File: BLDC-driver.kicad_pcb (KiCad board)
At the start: 2 copper layers, 55.9 x 56 mm, 60 parts, among them J1 Conn_01x06, J2 Conn_01x06, Q1 FDMS86550, Q2 FDMS86550, Q3 FDMS86550, Q4 FDMS86550, Q5 FDMS86550, Q6 FDMS86550, U1 ADP3120A, U2 STM32F103C8Tx, U3 AS5600, U4 ADP3120A, U5 ADP3120A, U6 MP2359, U7 MIC5504-3.3YM5

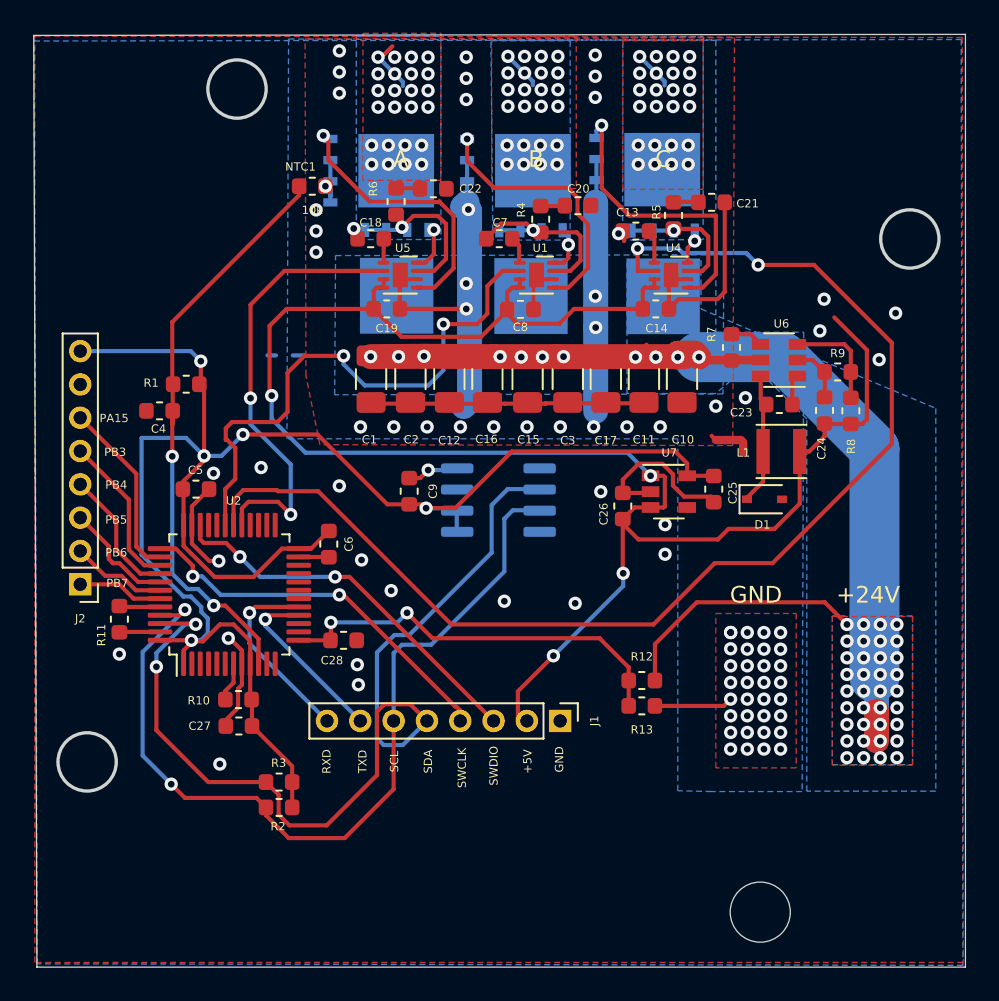
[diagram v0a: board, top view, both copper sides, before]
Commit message: Latest
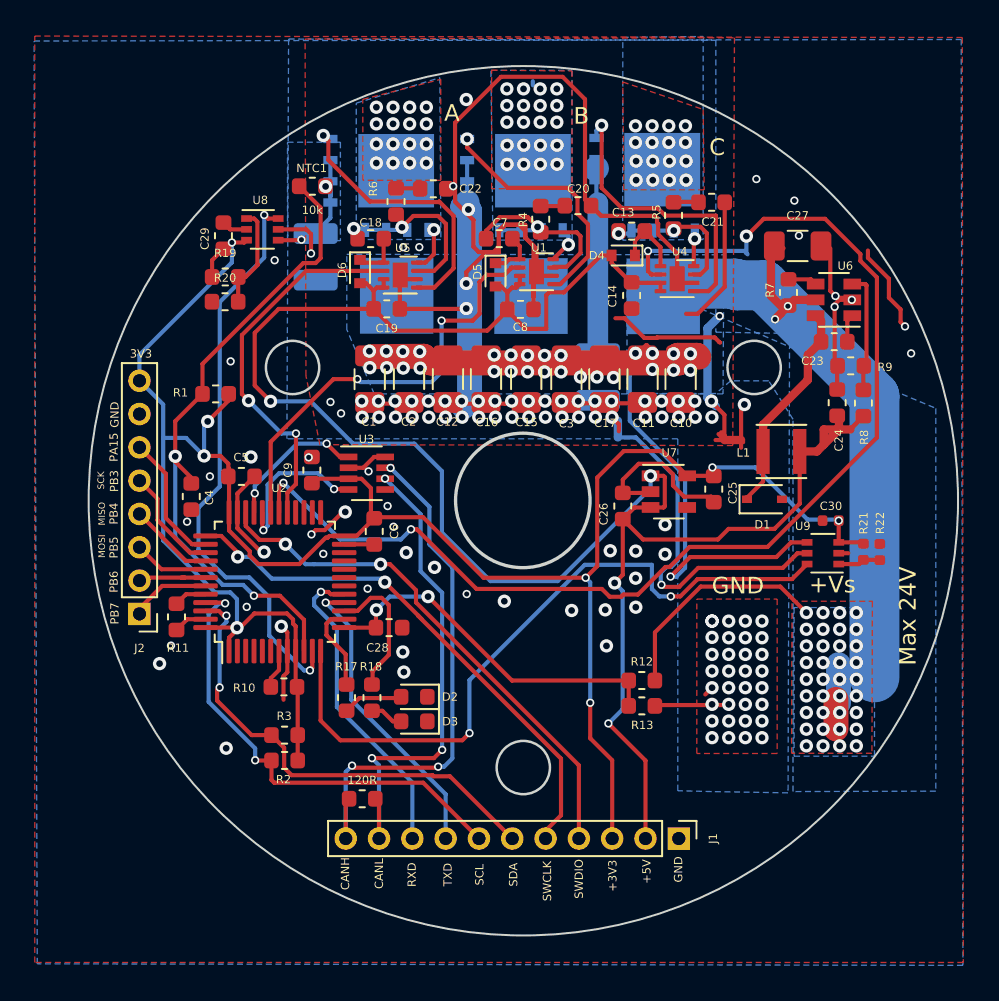
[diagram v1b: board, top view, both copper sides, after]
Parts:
- added C29: 100nF, Capacitor_SMD:C_0603_1608Metric, F.Cu at (178.7, 107.2)
- added C30: 100nF, Capacitor_SMD:C_0402_1005Metric, F.Cu at (215.2, 124.3)
- added D2: LED, LED_SMD:LED_0603_1608Metric, F.Cu at (190.2, 134.9)
- added D3: LED, LED_SMD:LED_0603_1608Metric, F.Cu at (190.2, 136.4)
- added D4: 30V, Diode_SMD:D_SOD-523, F.Cu at (202.7, 108.4)
- added D5: 30V, Diode_SMD:D_SOD-523, F.Cu at (195.0, 109.6)
- added D6: 30V, Diode_SMD:D_SOD-523, F.Cu at (186.9, 109.4)
- added NT2: Net-Tie_2, NetTie:NetTie-2_SMD_Pad0.5mm, B.Cu at (202.4, 118.8)
- added R14: 0.001, Resistor_SMD:R_1210_3225Metric, B.Cu at (184.3, 108.5)
- added R15: 0.001, Resistor_SMD:R_1210_3225Metric, B.Cu at (201.2, 115.7)
- added R16: 120R, Resistor_SMD:R_0603_1608Metric, F.Cu at (187.0, 141.0)
- added R17: 1k, Resistor_SMD:R_0603_1608Metric, F.Cu at (186.1, 135.0)
- added R18: 1k, Resistor_SMD:R_0603_1608Metric, F.Cu at (187.6, 135.0)
- added R19: 10k, Resistor_SMD:R_0603_1608Metric, F.Cu at (178.8, 109.7)
- added R20: 10k, Resistor_SMD:R_0603_1608Metric, F.Cu at (178.8, 111.2)
- added R21: 10k, Resistor_SMD:R_0402_1005Metric, F.Cu at (217.1, 126.2)
- added R22: 10k, Resistor_SMD:R_0402_1005Metric, F.Cu at (218.1, 126.2)
- added U8: NCS210, Package_TO_SOT_SMD:SOT-363_SC-70-6, F.Cu at (181.1, 106.8)
- added U9: NCS210, Package_TO_SOT_SMD:SOT-363_SC-70-6, F.Cu at (214.7, 126.3)
- C27: value 100nF -> 4.7uF; footprint Capacitor_SMD:C_0603_1608Metric -> Capacitor_SMD:C_1206_3216Metric
- J1: footprint Connector_PinHeader_2.00mm:PinHeader_1x08_P2.00mm_Vertical -> Connector_PinHeader_2.00mm:PinHeader_1x11_P2.00mm_Vertical
- U3: value AS5600 -> MAX3051; footprint Package_SO:SOIC-8_3.9x4.9mm_P1.27mm -> Package_TO_SOT_SMD:SOT-23-8; moved to F.Cu
- moved C27 44.2 mm to (213.2, 107.8)
- moved J1 10.0 mm to (206.1, 143.4)
- moved U3 8.06 mm to (187.3, 121.5)
- moved C9 5.98 mm to (184.0, 121.3), turned to 90 degrees
- moved C4 5.48 mm to (176.8, 122.9), turned to 90 degrees
- moved C23 5.01 mm to (215.4, 113.6)
- moved U6 4.90 mm to (215.4, 111.1)
- moved R7 4.75 mm to (212.6, 110.6)
- moved J2 3.98 mm to (173.7, 129.9)
- moved R11 3.43 mm to (175.9, 130.1)
- moved R2 2.84 mm to (182.4, 138.7)
- moved R3 2.84 mm to (182.4, 137.2)
- moved C28 2.83 mm to (188.7, 130.7)
- moved C5 2.83 mm to (179.8, 121.7)
- moved C6 2.83 mm to (187.8, 125.0)
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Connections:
- C27 pad 1: GND -> +24V
- C27 pad 2: +3V3 -> GND
- C9 pad 1: GND -> +3V3
- C9 pad 2: +3V3 -> GND
- J1 pad 3: /SWDIO -> +3V3
- J1 pad 4: /SWCLK -> /SWDIO
- J1 pad 5: /SDA -> /SWCLK
- J1 pad 6: /SCL -> /SDA
- J1 pad 7: /TXD -> /SCL
- J1 pad 8: /RXD -> /TXD
- NTC1 pad 2: GNDPWR -> /SH_C
- Q4 pad 1: GNDPWR -> /SH_B
- Q4 pad 2: GNDPWR -> /SH_B
- Q4 pad 3: GNDPWR -> /SH_B
- Q6 pad 1: GNDPWR -> /SH_C
- Q6 pad 2: GNDPWR -> /SH_C
- Q6 pad 3: GNDPWR -> /SH_C
- U2 pad 11: Net-(U2-Pad11) -> /CURR_C
- U2 pad 12: Net-(U2-Pad12) -> /CURR_B
- U2 pad 14: Net-(U2-Pad14) -> /LEDR
- U2 pad 15: Net-(U2-Pad15) -> /LEDG
- U2 pad 32: Net-(U2-Pad32) -> /CANRX
- U2 pad 33: Net-(U2-Pad33) -> /CANTX
- U3 pad 1: +3V3 -> /CANTX
- U3 pad 2: +3V3 -> GND
- U3 pad 3: Net-(U3-Pad3) -> +3V3
- U3 pad 4: GND -> /CANRX
- U3 pad 5: Net-(U3-Pad5) -> GND
- U3 pad 6: /SDA -> /CANL
- U3 pad 7: /SCL -> /CANH
- U3 pad 8: Net-(U3-Pad8) -> GND
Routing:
- net GNDPWR: track 79.9 -> 130.2 mm, vias 62 -> 86
- net /CURR_B: track 0.00 -> 42.5 mm, vias 0 -> 2
- net /SH_B: track 0.00 -> 37.4 mm, vias 0 -> 1
- net /CURR_C: track 0.00 -> 34.9 mm, vias 0 -> 2
- net /CANH: track 0.00 -> 32.6 mm, vias 0 -> 3
- net /SDA: track 59.3 -> 28.6 mm
- net /CANL: track 0.00 -> 29.6 mm, vias 0 -> 3
- net +3V3: track 106.5 -> 134.9 mm, vias 5 -> 8
- net /SCL: track 52.4 -> 28.5 mm
- net Net-(NT2-Pad2): track 0.00 -> 21.2 mm, vias 0 -> 1
- net GND: track 33.8 -> 50.2 mm, vias 22 -> 43
- net +5V: track 109.8 -> 123.6 mm
- net /CANRX: track 0.00 -> 9.47 mm, vias 0 -> 2
- net /SWCLK: track 23.1 -> 32.3 mm
- net /CANTX: track 0.00 -> 8.62 mm, vias 0 -> 2
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- added copper zone on B.Cu, net /SH_C
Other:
- board size 55.9 x 56 mm -> 52.2 x 52.2 mm
- board text added: "+3V3"
- board text added: "+Vs"
- board text added: "3V3"
- board text added: "CANH"
- board text added: "CANL"
- board text added: "MISO"
- board text added: "MOSI"
- board text added: "Max 24V"
- board text added: "SCK"
- board text removed: "+24V"
